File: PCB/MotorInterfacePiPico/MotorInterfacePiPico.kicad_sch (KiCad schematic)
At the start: 1 part, among them U1 RP2040

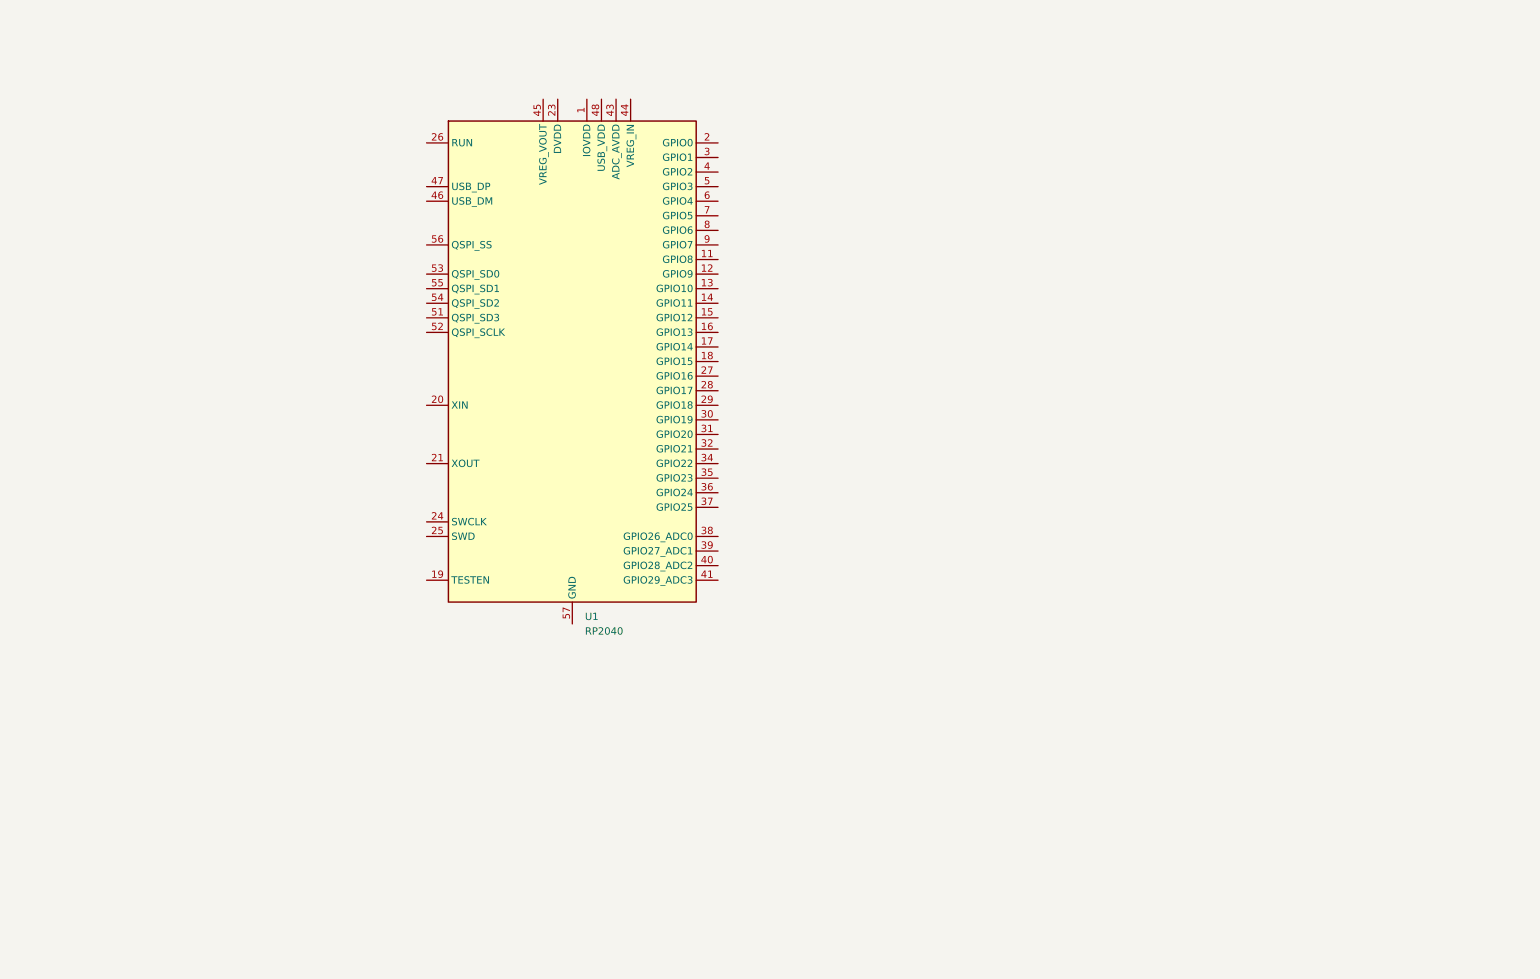
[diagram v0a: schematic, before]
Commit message: schema nearly finished
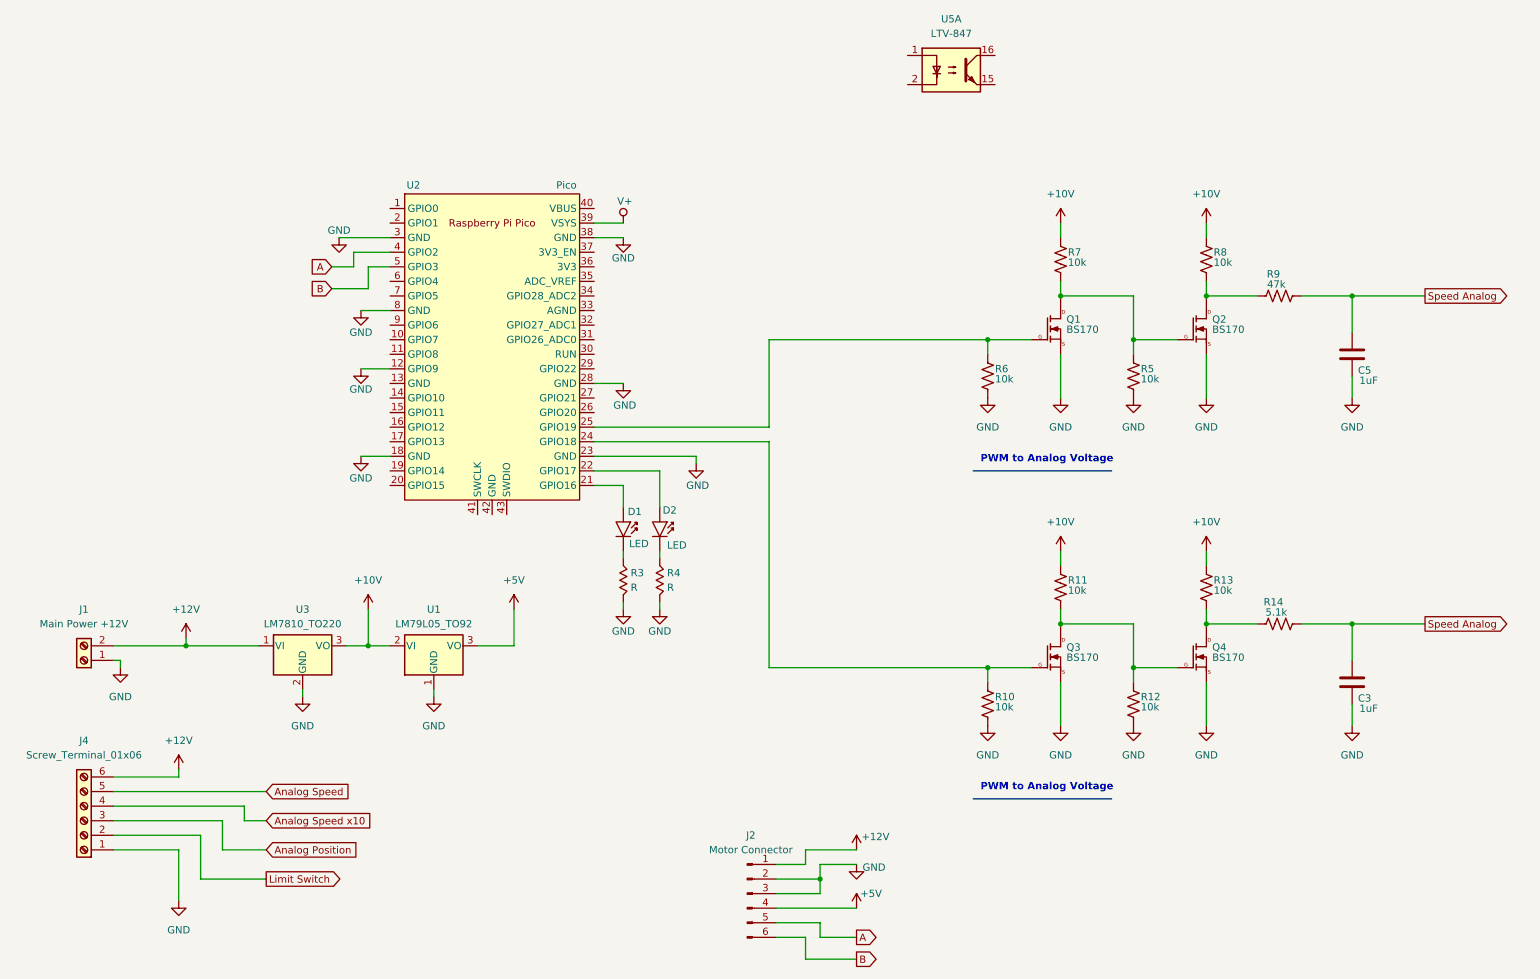
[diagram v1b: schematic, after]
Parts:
- removed U1: RP2040, Package_DFN_QFN:QFN-56-1EP_7x7mm_P0.4mm_EP3.2x3.2mm, symbol MCU_RaspberryPi:RP2040
- added C3, C5: 1uF, symbol F2018-cache:C
- added D1, D2: LED, symbol 00TJR:LED
- added J1: Main Power +12V, symbol Connector:Screw_Terminal_01x02
- added J2: Motor Connector, symbol Connector:Conn_01x06_Pin
- added J4: Screw_Terminal_01x06, symbol Connector:Screw_Terminal_01x06
- added Q1, Q2, Q3, Q4: BS170, Package_TO_SOT_THT:TO-92_Inline, symbol 00TJR:BS170_copy
- added R10, R11, R12, R13, R5, R6, R7, R8: 10k, symbol S2020-cache:Device_R_US
- added R14: 5.1k, symbol S2020-cache:Device_R_US
- added R3, R4: R, symbol 00TJR:R
- added R9: 47k, symbol S2020-cache:Device_R_US
- added U1: LM79L05_TO92, Package_TO_SOT_THT:TO-92_Inline, symbol Regulator_Linear:LM79L05_TO92
- added U2: Pico, RPi_Pico:RPi_Pico_SMD_TH, symbol MCU_RaspberryPi_and_Boards:Pico
- added U3: LM7810_TO220, Package_TO_SOT_THT:TO-220-3_Vertical, symbol Regulator_Linear:LM7810_TO220
- added U5: LTV-847, Package_DIP:DIP-16_W7.62mm, symbol Isolator:LTV-847
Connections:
- new net: Q2.1 (D), R8.2, R9.1
- new net: Q1.1 (D), Q2.2 (G), R5.1, R7.2
- new net: Q3.1 (D), Q4.2 (G), R11.2, R12.1
- new net: Q4.1 (D), R13.2, R14.1
- new net: Q1.2 (G), R6.1, U2.25 (GPIO19)
- new net: D1.2 (A), U2.21 (GPIO16)
- new net: D2.2 (A), U2.22 (GPIO17)
- new net: Q3.2 (G), R10.1, U2.24 (GPIO18)
- new net: D2.1 (K), R4.1
- new net: D1.1 (K), R3.1
- new net +10V: R11.1, R13.1, R7.1, R8.1, U1.2 (VI), U3.3 (VO)
- new net +12V: J1.2 (Pin_2), J2.1 (Pin_1), J4.6 (Pin_6), U3.1 (VI)
- new net +5V: J2.4 (Pin_4), U1.3 (VO)
- new net A: J2.5 (Pin_5), U2.4 (GPIO2)
- new net Analog Position: J4.3 (Pin_3)
- new net Analog Speed: J4.5 (Pin_5)
- new net Analog Speed x10: J4.4 (Pin_4)
- new net B: J2.6 (Pin_6), U2.5 (GPIO3)
- new net GND: C3.2, C5.2, J1.1 (Pin_1), J2.2 (Pin_2), J2.3 (Pin_3), J4.1 (Pin_1), Q1.3 (S), Q2.3 (S), Q3.3 (S), Q4.3 (S), R10.2, R12.2, R3.2, R4.2, R5.2, R6.2, U1.1 (GND), U2.12 (GPIO9), U2.18 (GND), U2.23 (GND), U2.28 (GND), U2.3 (GND), U2.38 (GND), U2.8 (GND), U3.2 (GND)
- new net Limit Switch: J4.2 (Pin_2)
- new net Speed Analog: C3.1, C5.1, R14.2, R9.2
- new net V+: U2.39 (VSYS)
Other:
- note added: "PWM to Analog Voltage"
